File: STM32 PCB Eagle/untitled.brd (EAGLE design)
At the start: 48.2 x 58.1 mm, 14 parts, among them IC1 LTV-846S, U1 SN65HVD230/1

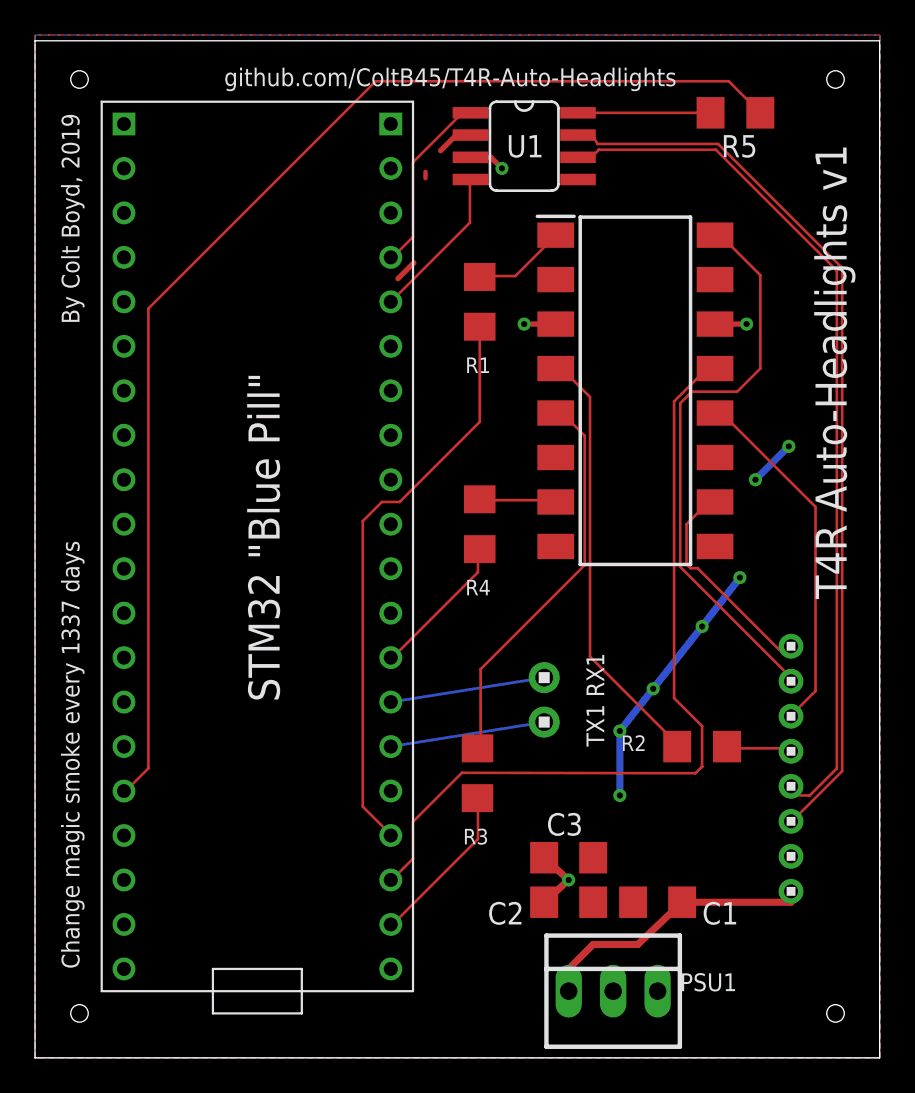
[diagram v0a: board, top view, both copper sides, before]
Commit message: This is the version sent to printing.
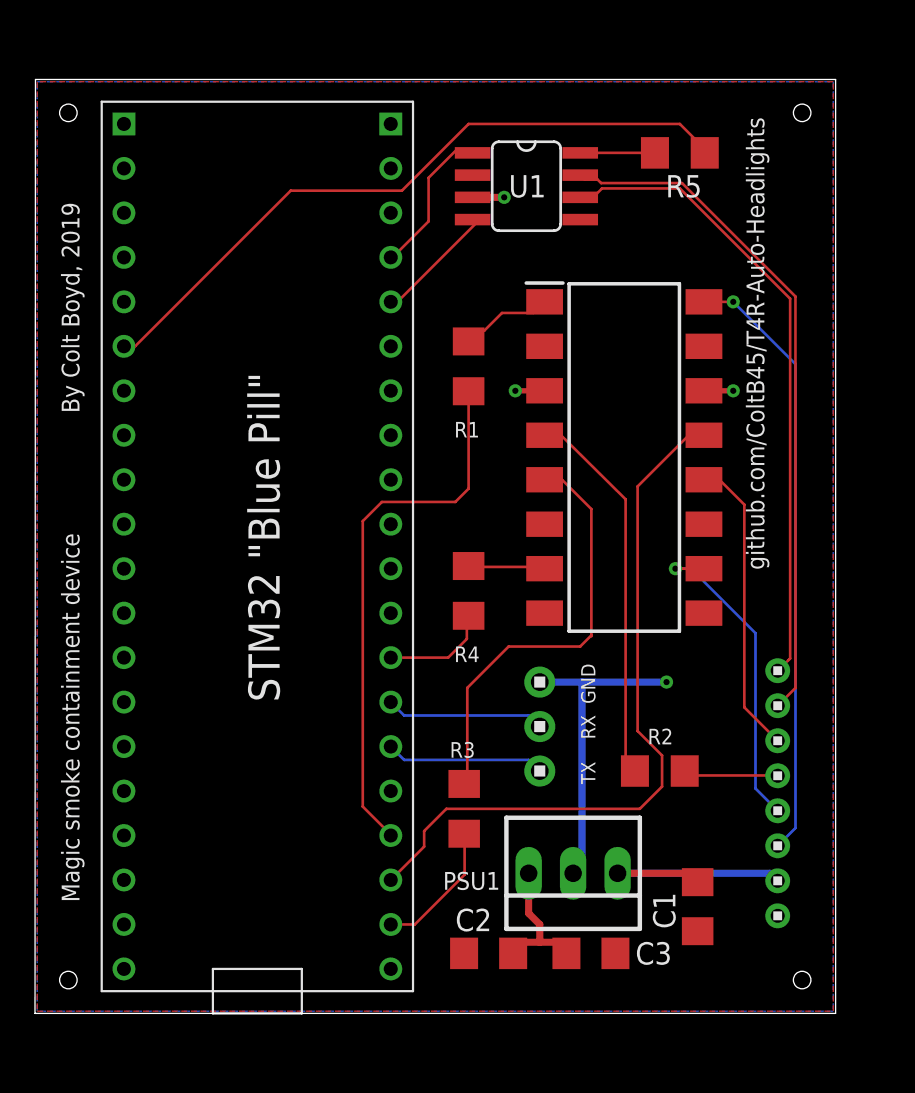
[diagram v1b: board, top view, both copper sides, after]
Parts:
- H1: value 1X2 -> 1X3; device headers(.1in):1X2 -> headers(.1in):1X3
- moved PSU1 7.11 mm to (30.7, 10.5), turned to 180 degrees
- moved C3 5.61 mm to (31.8, 5.97)
- moved C2 5.43 mm to (25.9, 5.97), turned to 0 degrees
- moved R5 3.91 mm to (36.8, 51.7)
- moved IC1 3.86 mm to (33.7, 34.3)
- moved R4 3.86 mm to (24.8, 26.7)
- moved R1 3.74 mm to (24.8, 39.5)
- moved H1 2.81 mm to (28.8, 16.4)
- moved R2 2.79 mm to (35.7, 16.4)
- moved C1 2.30 mm to (37.8, 8.64), turned to 270 degrees
- moved U1 2.29 mm to (28.1, 49.8)
- moved R3 2.17 mm to (24.5, 14.2)
- moved U$1 1.59 mm to (42.4, 15.1)
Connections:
- new net PA1: R5.1, STM32.P$6
- net 12V: now also U$1.2; no longer U$1.1
- net CANH: now also U$1.7; no longer U$1.3
- net CANL: now also U$1.8; no longer U$1.4
- net GND: now also H1.3, U$1.1; no longer U$1.2
- net HDL_MPX: now also U$1.3; no longer U$1.7
- net PB11: no longer R5.1
- net TL_MPX: now also U$1.4; no longer U$1.8
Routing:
- net PB11: track 69.3 -> 0.00 mm
- net PA1: track 0.00 -> 39.3 mm
- net CANL: track 50.0 -> 36.4 mm
- net CANH: track 51.1 -> 39.0 mm
- net PB14: track 46.3 -> 40.9 mm
- net TL_MPX: track 13.1 -> 18.4 mm, vias 0 -> 1
- net DRL_MPX: track 21.3 -> 17.2 mm
- net 3V3: track 9.45 -> 12.9 mm, vias 4 -> 3
- net GND: track 21.7 -> 18.4 mm, vias 7 -> 1
- net N$9: track 7.57 -> 4.27 mm
- net N$4: track 24.6 -> 22.2 mm
- net PA11: track 8.36 -> 6.15 mm
- net 12V: track 16.2 -> 14.1 mm
- net PB15: track 33.2 -> 31.1 mm
- net N$6: track 22.6 -> 24.5 mm
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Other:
- board size 48.2 x 58.1 mm -> 45.7 x 53.3 mm
- board text added: "Magic smoke containment device"
- board text added: "TX RX GND"
- board text removed: "Change magic smoke every 1337 days"
- board text removed: "T4R Auto-Headlights v1"
- board text removed: "TX1 RX1"
